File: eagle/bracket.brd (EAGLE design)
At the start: 39.3 x 38.1 mm, 15 parts, among them IC1 MAX6520, Q1 MMBT2222A, U1 GP-2106

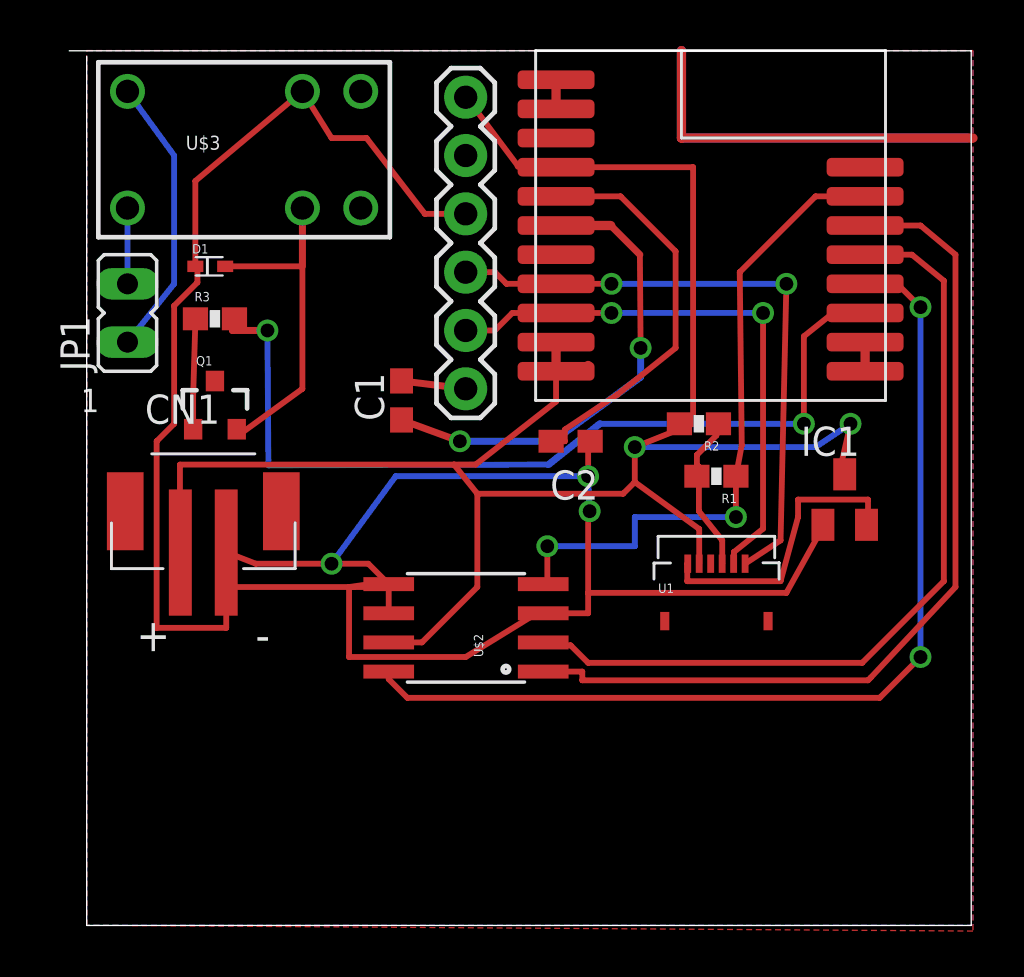
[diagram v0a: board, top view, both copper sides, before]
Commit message: updating board
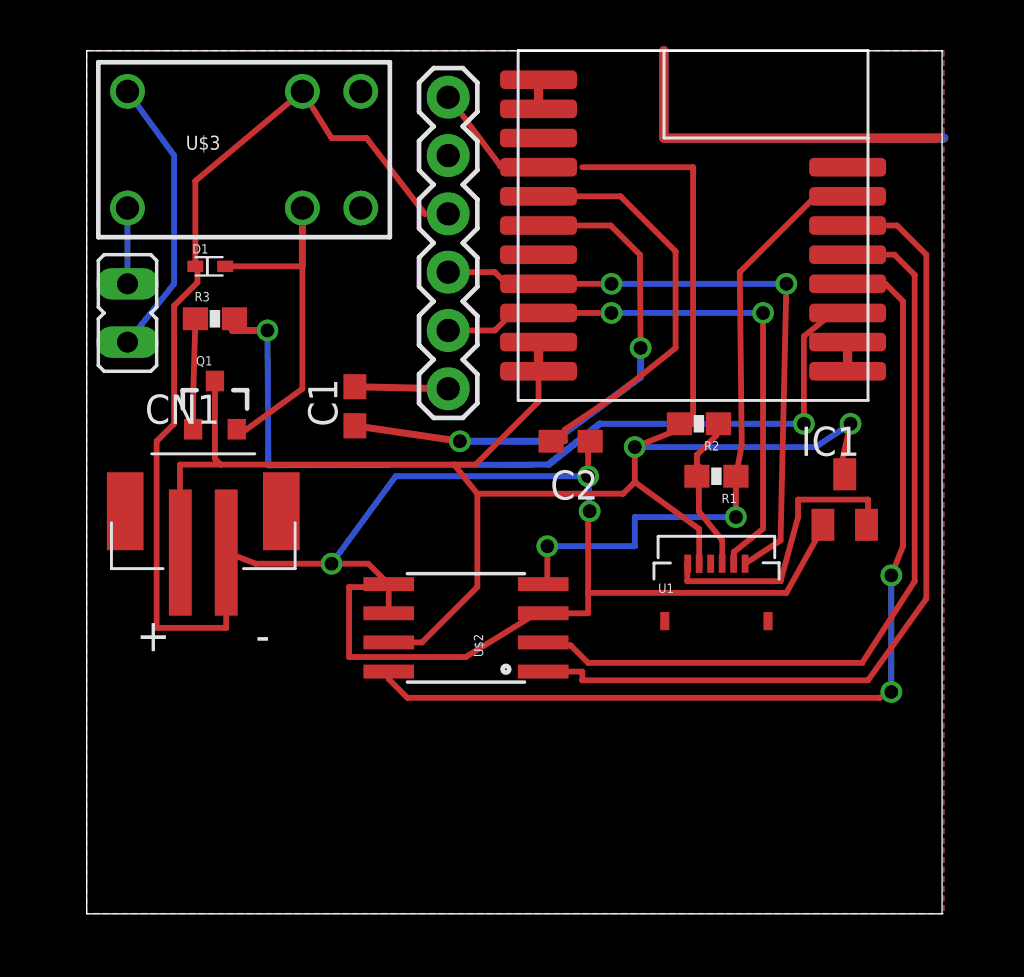
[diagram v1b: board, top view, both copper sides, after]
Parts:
- moved C1 2.05 mm to (46.0, 50.5)
- moved JP2 0.76 mm to (50.0, 51.3)
- moved U$1 0.76 mm to (60.7, 58.4)
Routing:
- net N$26: track 7.11 -> 0.00 mm
- net GND: track 86.9 -> 89.6 mm
- net N$6: track 21.0 -> 23.7 mm
- net N$7: track 2.81 -> 4.06 mm
- net N$9: track 39.0 -> 37.8 mm
- net N$14: track 36.3 -> 35.2 mm
- net VCC: track 86.1 -> 85.3 mm
- net N$8: track 27.2 -> 28.0 mm
- net N$2: track 16.5 -> 15.7 mm
- net N$19: track 17.5 -> 18.3 mm
- net N$18: track 28.8 -> 28.1 mm
- net N$1: track 24.8 -> 25.6 mm
- net N$5: track 1.40 -> 1.91 mm
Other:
- board size 39.3 x 38.1 mm -> 37.3 x 37.6 mm
- board text removed: "1"
